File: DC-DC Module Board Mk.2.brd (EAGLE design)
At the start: 177.9 x 101.7 mm, 151 parts, among them T1 FDN340P, T2 AP1117_LIN_REG, U3 LM1085IS-5.0

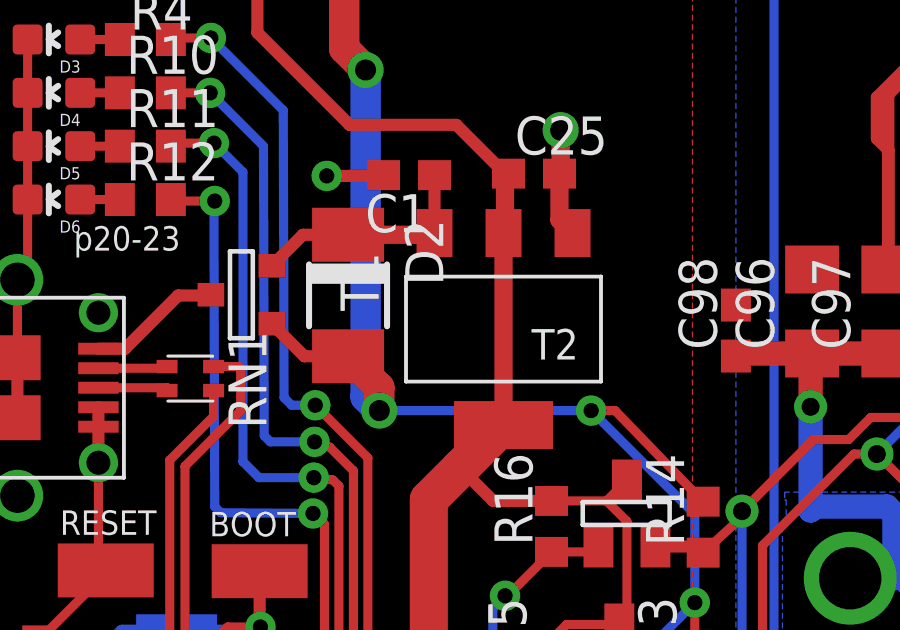
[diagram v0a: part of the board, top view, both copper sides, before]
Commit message: many aesthetic corrections
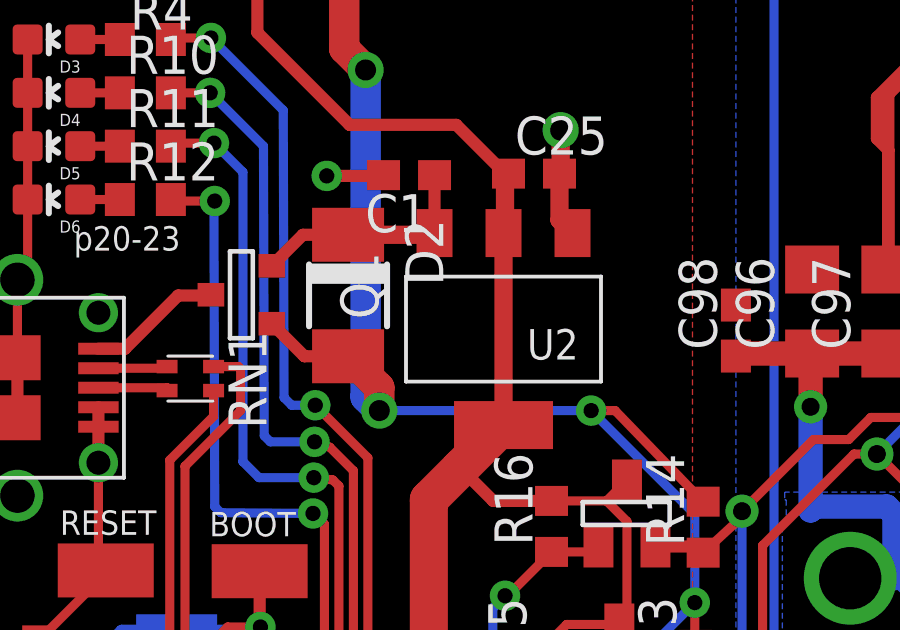
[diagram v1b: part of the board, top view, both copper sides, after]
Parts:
- C14, C15, C16: value .1u -> .1uF
- C19, C20: value 15u -> 15uF
- C21: value 10u -> 10uF
- renumbered T1 to Q1, T2 to U2, U$7 to J$7
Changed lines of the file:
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@@
 <attribute name="BOM" value="INCLUDE" x="95.25" y="80.01" size="1.778" layer="27" rot="R90" display="off"/>
 </element>
-<element name="C19" library="rcl" package="C3216" value="15u" x="87.63" y="91.44" rot="R90"/>
-<element name="C20" library="rcl" package="C3216" value="15u" x="90.17" y="91.44" rot="R90"/>
-<element name="C21" library="rcl" package="C0603" value="10u" x="85.09" y="90.805" rot="R90"/>
-<element name="C14" library="rcl" package="C0603" value=".1u" x="133.35" y="92.71" rot="R270"/>
-<element name="C15" library="rcl" package="C0603" value=".1u" x="130.81" y="92.71" rot="R270"/>
-<element name="C16" library="rcl" package="C0603" value=".1u" x="127" y="92.71" rot="R270"/>
+<element name="C19" library="rcl" package="C3216" value="15uF" x="87.63" y="91.44" rot="R90"/>
+<element name="C20" library="rcl" package="C3216" value="15uF" x="90.17" y="91.44" rot="R90"/>
+<element name="C21" library="rcl" package="C0603" value="10uF" x="85.09" y="90.805" rot="R90"/>
+<element name="C14" library="rcl" package="C0603" value=".1uF" x="133.35" y="92.71" rot="R270"/>
+<element name="C15" library="rcl" package="C0603" value=".1uF" x="130.81" y="92.71" rot="R270"/>
+<element name="C16" library="rcl" package="C0603" value=".1uF" x="127" y="92.71" rot="R270"/>
 <element name="U$2" library="Connectors" package="XT60" value="XT60" x="95.25" y="54.61" rot="R90"/>
 <element name="C22" library="ux-capacitor" package="NICHICON-UX-8X10" value="10uF" x="120.65" y="91.44"/>
@@
 <attribute name="BOM" value="INCLUDE" x="140.97" y="2.54" size="1.778" layer="27" rot="R90" display="off"/>
 </element>
-<element name="U$7" library="Other" package="MICRO_B" value="MICROUSB" x="0" y="33.02" rot="R270"/>
+<element name="J$7" library="Other" package="MICRO_B" value="MICROUSB" x="0" y="33.02" rot="R270"/>
 <element name="RN1" library="DiscreteComponents" package="EXBV4V" value="" x="7.2136" y="33.3248" rot="R270">
 <attribute name="MPN" value="MNR12ERAPJ220" x="22.4536" y="42.2148" size="1.778" layer="27" rot="R270" display="off"/>
@@
 <attribute name="DIGIKEY" value="RHM1381CT-ND" x="22.4536" y="42.2148" size="1.778" layer="27" rot="R270" display="off"/>
 </element>
-<element name="T1" library="DiscreteComponents" package="SOT-23" value="FDN340P" x="8.9154" y="36.1442" rot="R270">
+<element name="Q1" library="DiscreteComponents" package="SOT-23" value="FDN340P" x="8.9154" y="36.1442" rot="R270">
 <attribute name="DIGIKEY" value="FDN340PCT-ND" x="6.3754" y="36.1442" size="1.778" layer="27" rot="R270" display="off"/>
 </element>
 <element name="D2" library="DiscreteComponents" package="DO-214AC" value="" x="12.4714" y="36.0934" rot="R270"/>
-<element name="T2" library="PowerComponents" package="SOT223" value="AP1117_LIN_REG" x="17.653" y="34.9758" rot="R180"/>
+<element name="U2" library="PowerComponents" package="SOT223" value="AP1117_LIN_REG" x="17.653" y="34.9758" rot="R180"/>
 <element name="C1" library="rcl" package="C0603" value="0.22uF" x="14.5034" y="40.1066" rot="R180"/>
 <element name="C25" library="rcl" package="C0603" value="0.22uF" x="18.669" y="40.1574"/>
@@
 <contactref element="C25" pad="2"/>
 <contactref element="C1" pad="2"/>
-<contactref element="T2" pad="GND"/>
-<contactref element="U$7" pad="P5"/>
-<contactref element="U$7" pad="GND3"/>
-<contactref element="U$7" pad="GND1"/>
-<contactref element="U$7" pad="GND4"/>
-<contactref element="U$7" pad="GND7"/>
-<contactref element="U$7" pad="GND2"/>
-<contactref element="U$7" pad="GND8"/>
-<contactref element="U$7" pad="P4"/>
+<contactref element="U2" pad="GND"/>
+<contactref element="J$7" pad="P5"/>
+<contactref element="J$7" pad="GND3"/>
+<contactref element="J$7" pad="GND1"/>
+<contactref element="J$7" pad="GND4"/>
+<contactref element="J$7" pad="GND7"/>
+<contactref element="J$7" pad="GND2"/>
+<contactref element="J$7" pad="GND8"/>
+<contactref element="J$7" pad="P4"/>
 <contactref element="U$8" pad="2"/>
 <contactref element="R17" pad="1"/>
@@
 <contactref element="U$8" pad="3"/>
 <contactref element="C25" pad="1"/>
-<contactref element="T2" pad="VOUT"/>
-<contactref element="T2" pad="TAB"/>
+<contactref element="U2" pad="VOUT"/>
+<contactref element="U2" pad="TAB"/>
 <contactref element="R21" pad="2"/>
 <contactref element="R30" pad="2"/>
@@
 <contactref element="D10" pad="1"/>
 <contactref element="C29" pad="2"/>
-<contactref element="T1" pad="3"/>
+<contactref element="Q1" pad="3"/>
 <contactref element="D2" pad="A"/>
 <contactref element="U$30" pad="C2"/>
@@
 </signal>
 <signal name="N$24">
-<contactref element="U$7" pad="P3"/>
+<contactref element="J$7" pad="P3"/>
 <contactref element="RN1" pad="2"/>
 <wire x1="4.15" y1="33.02" x2="6.4386" y2="33.02" width="0.3048" layer="1"/>
@@
 </signal>
 <signal name="N$57">
-<contactref element="U$7" pad="P1"/>
-<contactref element="T1" pad="1"/>
+<contactref element="J$7" pad="P1"/>
+<contactref element="Q1" pad="1"/>
 <wire x1="4.15" y1="34.32" x2="5.0338" y2="34.32" width="0.4064" layer="1"/>
 <wire x1="5.0338" y1="34.32" x2="6.8072" y2="36.0934" width="0.4064" layer="1"/>
@@
 <signal name="N$58">
 <contactref element="D2" pad="C"/>
-<contactref element="T1" pad="2"/>
-<contactref element="T2" pad="VIN"/>
+<contactref element="Q1" pad="2"/>
+<contactref element="U2" pad="VIN"/>
 <contactref element="C1" pad="1"/>
 <wire x1="12.4714" y1="38.1184" x2="10.9658" y2="38.1184" width="0.4064" layer="1"/>
@@
 <signal name="N$9">
 <contactref element="RN1" pad="1"/>
-<contactref element="U$7" pad="P2"/>
+<contactref element="J$7" pad="P2"/>
 <wire x1="4.15" y1="33.67" x2="6.4386" y2="33.67" width="0.3048" layer="1"/>
 <wire x1="6.4386" y1="33.67" x2="6.4386" y2="33.7248" width="0.3048" layer="1"/>
